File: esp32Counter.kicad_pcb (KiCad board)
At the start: 2 copper layers, 82.5 x 43.2 mm, 20 parts, among them J1 Jack-DC, J2 USB<->ttl, J3 SPI_CONN, J4 GPIO_5_4_0, SW1 SW_Push, SW2 SW_Push, U1 AMS1117-3.3, U2 ESP-07

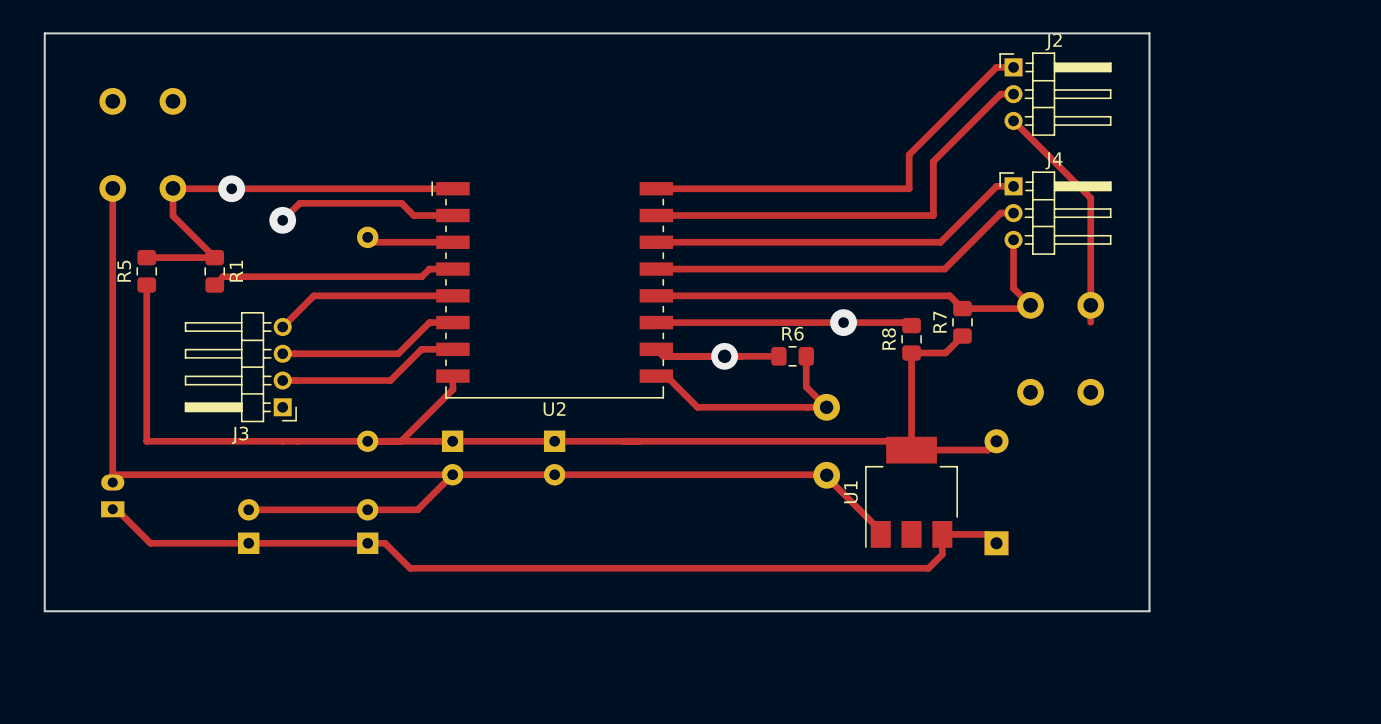
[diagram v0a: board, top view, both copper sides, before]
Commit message: v1.01
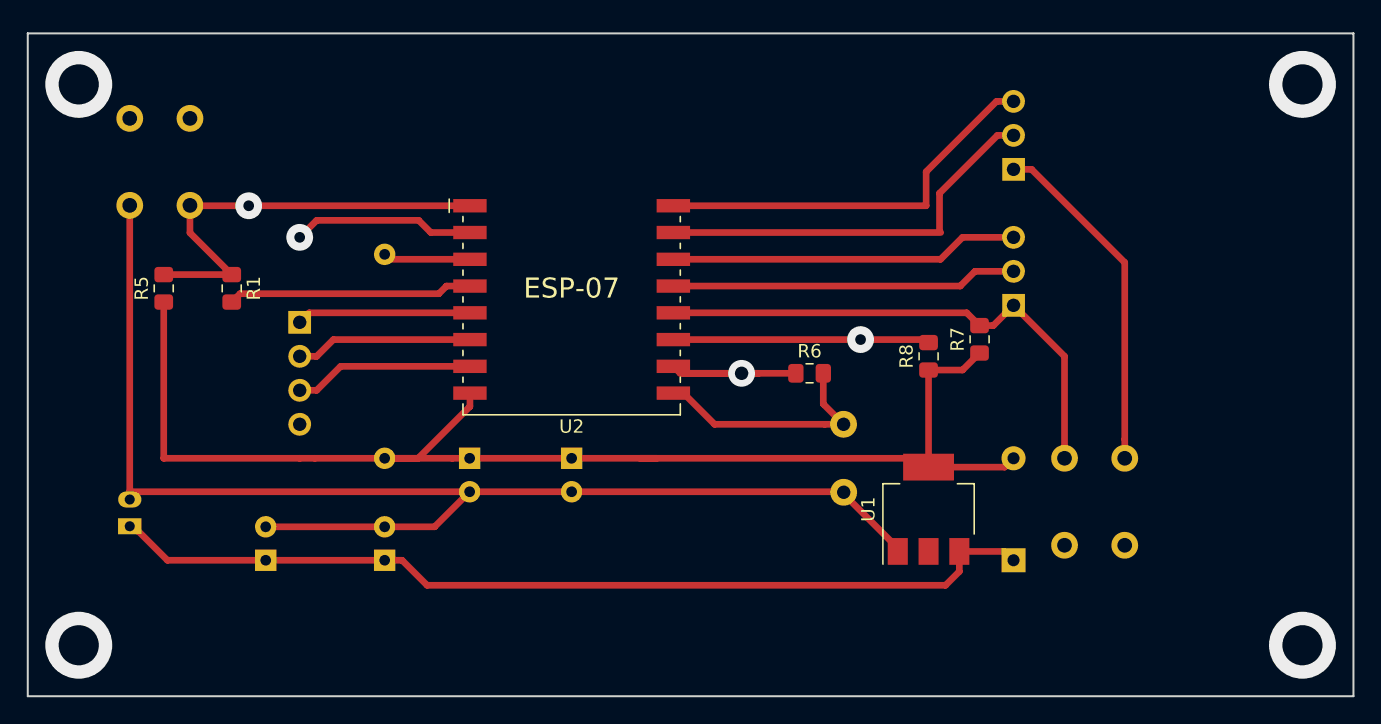
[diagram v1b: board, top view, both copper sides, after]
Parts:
- J2, J4: footprint Connector_PinHeader_2.00mm:PinHeader_1x03_P2.00mm_Horizontal -> Connector_PinHeader_2.54mm:PinHeader_1x03_P2.54mm_Horizontal; moved to B.Cu
- J3: footprint Connector_PinHeader_2.00mm:PinHeader_1x04_P2.00mm_Horizontal -> Connector_PinHeader_2.54mm:PinHeader_1x04_P2.54mm_Horizontal; moved to B.Cu
- moved SW2 11.7 mm to (90.2, 44.5)
- moved J4 8.89 mm to (86.4, 33.0)
- moved J2 7.62 mm to (86.4, 22.9)
- moved J3 6.48 mm to (33.0, 34.3)
- moved R6 1.80 mm to (71.1, 38.1)
- moved C4 1.80 mm to (53.3, 44.5)
- moved R8 1.80 mm to (80.0, 36.8)
- moved U1 1.80 mm to (80.0, 48.3)
- moved C3 1.80 mm to (30.5, 52.1)
- moved J1 1.80 mm to (20.3, 49.5)
- moved U2 1.80 mm to (53.3, 30.5)
- moved C1 1.80 mm to (39.4, 52.1)
- moved C2 1.80 mm to (45.7, 44.5)
- moved D1 1.80 mm to (86.4, 52.1)
- moved R1 1.80 mm to (27.9, 31.8)
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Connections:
- J2 pad 1: /TXtoRX -> Net-(J2-Pad1)
- J2 pad 3: Net-(J2-Pad3) -> /TXtoRX
- J3 pad 1: Net-(J3-Pad1) -> /HSPI_CLK
- J3 pad 2: /HSPI_MOSI -> /HSPI_MISO
- J3 pad 3: /HSPI_MISO -> /HSPI_MOSI
- J3 pad 4: /HSPI_CLK -> Net-(J3-Pad4)
- J4 pad 1: /GPIO5 -> /GIPO0
- J4 pad 3: /GIPO0 -> /GPIO5
- SW2 pad 2: Net-(J2-Pad3) -> Net-(J2-Pad1)
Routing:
- net Net-(J2-Pad1): track 0.00 -> 25.8 mm
- net Net-(J2-Pad3): track 17.4 -> 0.00 mm
- net /GIPO0: track 33.9 -> 39.5 mm
- net /RXtoTX: track 32.8 -> 30.1 mm
- net /GPIO4: track 28.4 -> 25.9 mm
- net /GPIO5: track 28.4 -> 26.1 mm
- net /TXtoRX: track 31.9 -> 30.1 mm
- net /HSPI_CLK: track 13.7 -> 13.0 mm
- net (no net): vias 0 -> 4
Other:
- board size 82.5 x 43.2 mm -> 99.1 x 49.5 mm
- board text added: "ESP-07"
